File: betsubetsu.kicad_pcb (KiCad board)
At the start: 2 copper layers, 64.5 x 39.4 mm, 24 parts, among them J1 AV IN, J2 VIDEO OUT, J3 AUDIO OUT, T1 TY-250P, U1 THS7374

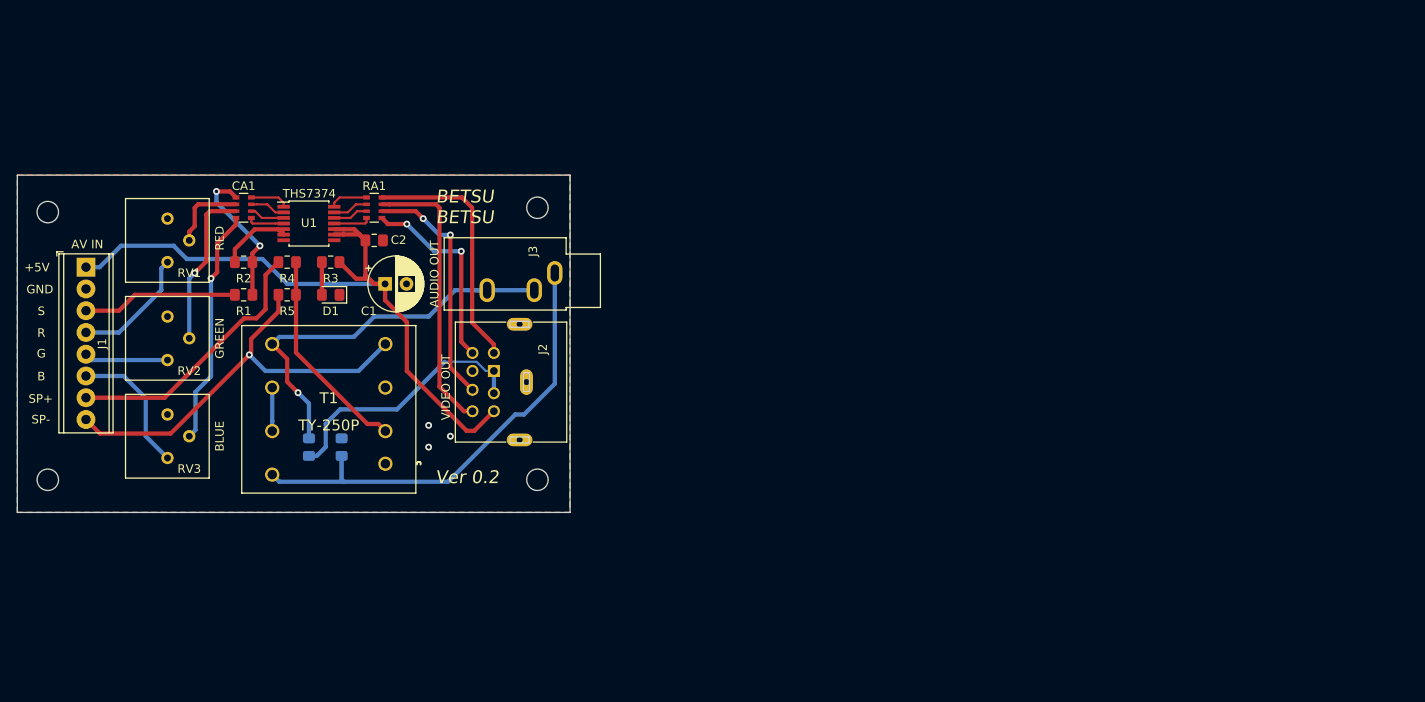
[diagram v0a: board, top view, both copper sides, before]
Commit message: Cleaned up jamma version
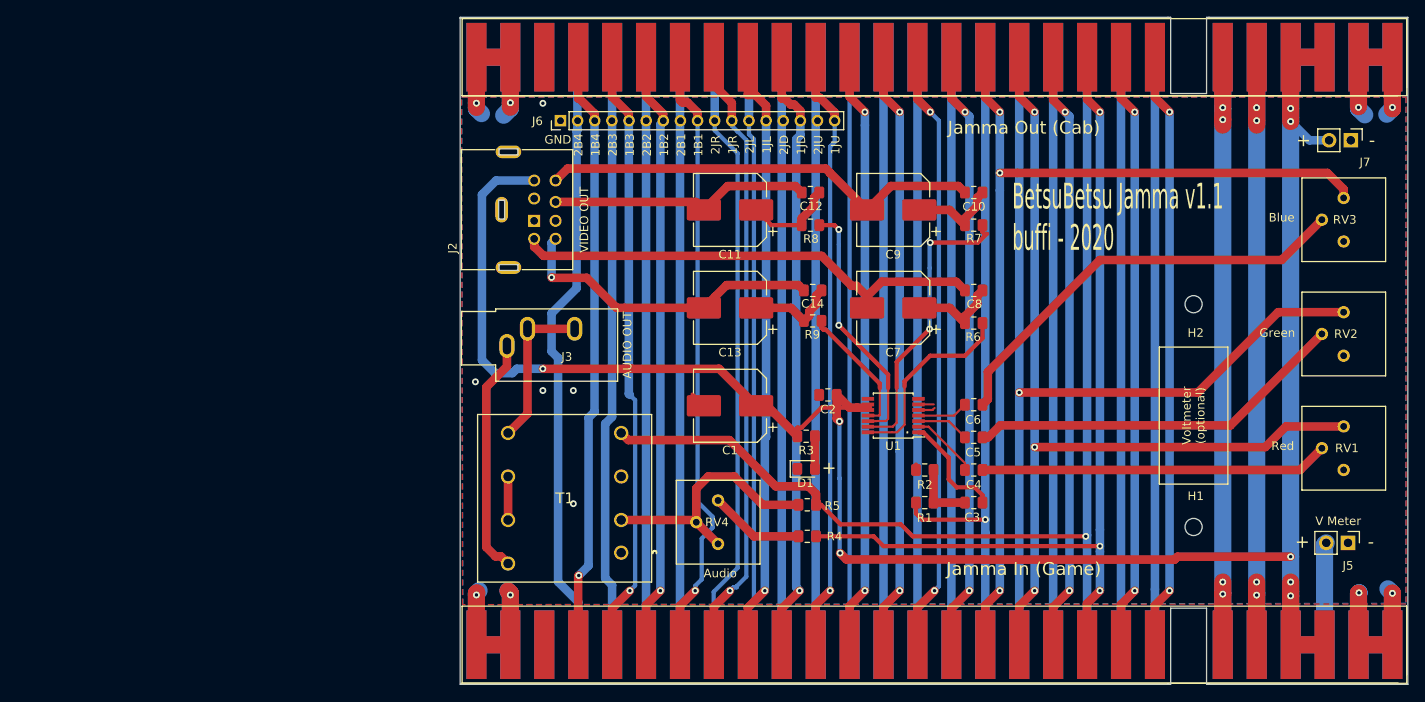
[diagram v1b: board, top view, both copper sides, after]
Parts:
- removed CA1: 0.1uF, Resistor_SMD:R_Array_Convex_4x0603
- removed H3, H4: MountingHole, MountingHole:MountingHole_2.5mm
- removed JMP1: SCART_AUDIO, LED_SMD:LED_0805_2012Metric_Pad1.15x1.40mm_HandSolder
- removed JMP2: AUDIO_GND_TO_GLOBAL_GND, Resistor_SMD:R_0805_2012Metric_Pad1.15x1.40mm_HandSolder
- removed RA1: 75, Resistor_SMD:R_Array_Convex_4x0603
- added C10: 0.1u, Capacitor_SMD:C_0805_2012Metric_Pad1.15x1.40mm_HandSolder, F.Cu at (156.3, 77.0)
- added C11: 470u, Capacitor_SMD:CP_Elec_8x6.7, F.Cu at (127.9, 79.0)
- added C12: 0.1u, Capacitor_SMD:C_0805_2012Metric_Pad1.15x1.40mm_HandSolder, F.Cu at (137.3, 77.0)
- added C13: 470u, Capacitor_SMD:CP_Elec_8x6.7, F.Cu at (127.9, 90.4)
- added C14: 0.1u, Capacitor_SMD:C_0805_2012Metric_Pad1.15x1.40mm_HandSolder, F.Cu at (137.5, 88.4)
- added C3: 0.1u, Capacitor_SMD:C_0805_2012Metric_Pad1.15x1.40mm_HandSolder, F.Cu at (156.3, 113.2)
- added C4: 0.1u, Capacitor_SMD:C_0805_2012Metric_Pad1.15x1.40mm_HandSolder, F.Cu at (156.3, 109.3)
- added C5: 0.1u, Capacitor_SMD:C_0805_2012Metric_Pad1.15x1.40mm_HandSolder, F.Cu at (156.3, 105.5)
- added C6: 0.1u, Capacitor_SMD:C_0805_2012Metric_Pad1.15x1.40mm_HandSolder, F.Cu at (156.3, 101.7)
- added C7: 470u, Capacitor_SMD:CP_Elec_8x6.7, F.Cu at (146.9, 90.4)
- added C8: 0.1u, Capacitor_SMD:C_0805_2012Metric_Pad1.15x1.40mm_HandSolder, F.Cu at (156.3, 88.4)
- added C9: 470u, Capacitor_SMD:CP_Elec_8x6.7, F.Cu at (146.9, 79.0)
- added J4: Jamma In (Game), jamma_connector:JAMMA-56, F.Cu at (150.7, 110.7)
- added J5: V Meter, Connector_PinHeader_2.54mm:PinHeader_1x02_P2.54mm_Vertical, F.Cu at (200.0, 117.9)
- added J6: Conn_01x17, Connector_PinHeader_2.00mm:PinHeader_1x17_P2.00mm_Vertical, F.Cu at (108.1, 68.6)
- added J7: 5V, Connector_PinHeader_2.54mm:PinHeader_1x02_P2.54mm_Vertical, F.Cu at (200.4, 70.9)
- added R6: 75, Resistor_SMD:R_0805_2012Metric_Pad1.15x1.40mm_HandSolder, F.Cu at (156.3, 92.2)
- added R7: 75, Resistor_SMD:R_0805_2012Metric_Pad1.15x1.40mm_HandSolder, F.Cu at (156.3, 80.8)
- added R8: 75, Resistor_SMD:R_0805_2012Metric_Pad1.15x1.40mm_HandSolder, F.Cu at (137.3, 80.8)
- added R9: 75, Resistor_SMD:R_0805_2012Metric_Pad1.15x1.40mm_HandSolder, F.Cu at (137.5, 91.9)
- added RV4: 500, Potentiometer_THT:Potentiometer_Bourns_3386P_Vertical, F.Cu at (126.5, 112.9)
- C1: value 100uF -> 100u; footprint Capacitor_THT:CP_Radial_D6.3mm_P2.50mm -> Capacitor_SMD:CP_Elec_8x6.7
- C2: value 0.1uF -> 0.1u
- H1, H2: value MountingHole -> V METER HOLE (2mm); footprint MountingHole:MountingHole_2.5mm -> MountingHole:MountingHole_2mm
- J1: value AV IN -> Jamma Out (Cab); footprint TerminalBlock_Phoenix:TerminalBlock_Phoenix_MPT-0,5-8-2.54_1x08_P2.54mm_Horizontal -> jamma_connector:JAMMA-56
- J2: footprint MD-80SM:CUI_MD-80SM -> MD-80SM-Connector:MD-80SM
- moved RV3 140.6 mm to (199.5, 77.6), turned to 180 degrees
- moved RV1 138.6 mm to (199.5, 104.3), turned to 180 degrees
- moved RV2 137.4 mm to (199.5, 90.9), turned to 180 degrees
- moved H2 134.2 mm to (182.0, 90.0)
- moved H1 133.9 mm to (182.0, 116.0)
- moved J1 107.3 mm to (150.7, 42.2), turned to 180 degrees
- moved R1 83.1 mm to (150.6, 113.2)
- moved R2 83.1 mm to (150.6, 109.3)
- moved U1 71.8 mm to (146.9, 103.0), turned to 180 degrees
- moved R4 68.6 mm to (136.9, 117.1), turned to 180 degrees
- moved R5 65.5 mm to (136.9, 113.4), turned to 180 degrees
- moved D1 59.1 mm to (136.8, 109.2), turned to 0 degrees
- moved R3 59.1 mm to (136.8, 105.4), turned to 180 degrees
- moved C2 55.9 mm to (139.3, 100.6), turned to 0 degrees
- moved C1 42.7 mm to (127.9, 101.9), turned to 180 degrees
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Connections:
- J1 pad 1: +5V -> GND
- J1 pad 3: SYNC_IN -> +5V
- J1 pad 4: RED_IN -> +5V
- J1 pad 5: GREEN_IN -> -5V
- J1 pad 6: BLUE_IN -> +12V
- J1 pad 8: -AUDIO_IN -> METER1
- J2 pad 1: SCART_AUDIO_OUT -> (no net)
- J2 pad 2: SCART_AUDIO_OUT -> (no net)
- R5 pad 2: Net-(R4-Pad2) -> Net-(R5-Pad2)
- T1 pad 2: Net-(R4-Pad2) -> Net-(R5-Pad2)
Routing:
- net +5V: track 83.0 -> 269.9 mm, vias 0 -> 8
- net GND: track 9.07 -> 142.4 mm, vias 3 -> 13
- net GREEN_IN: track 9.80 -> 110.3 mm, vias 0 -> 1
- net BLUE_IN: track 16.1 -> 111.9 mm, vias 0 -> 3
- net RED_IN: track 14.4 -> 107.1 mm, vias 0 -> 3
- net +12V: track 0.00 -> 80.6 mm, vias 0 -> 4
- net -5V: track 0.00 -> 80.6 mm, vias 0 -> 4
- net -AUDIO_IN: track 49.9 -> 128.8 mm
- net P1_D: track 0.00 -> 74.4 mm, vias 0 -> 1
- net P1_B: track 0.00 -> 73.8 mm, vias 0 -> 1
- net +AUDIO_IN: track 31.4 -> 103.5 mm, vias 0 -> 3
- net P1_A: track 0.00 -> 72.1 mm, vias 0 -> 1
- net P1_RIGHT: track 0.00 -> 72.0 mm, vias 0 -> 1
- net P2_D: track 0.00 -> 71.2 mm
- net P1_DOWN: track 0.00 -> 71.1 mm, vias 0 -> 1
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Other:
- board size 64.5 x 39.4 mm -> 110.6 x 77.9 mm
- board text added: "+"
- board text added: "-"
- board text added: "."
- board text added: "1B1"
- board text added: "1B2"
- board text added: "1B3"
- board text added: "1B4"
- board text added: "1JD"
- board text added: "1JL"
- board text added: "1JR"
- board text added: "1JU"
- board text added: "2B1"
- board text added: "2B2"
- board text added: "2B3"
- board text added: "2B4"
- board text added: "2JD"
- board text added: "2JL"
- board text added: "2JR"
- board text added: "2JU"
- board text added: "Audio"
- board text added: "BetsuBetsu Jamma v1.1 buffi - 2020"
- board text added: "Blue"
- board text added: "Green"
- board text added: "Jamma In (Game)"
- board text added: "Jamma Out (Cab)"
- board text added: "Red"
- board text added: "Voltmeter (optional)"
- board text removed: "+5V"
- board text removed: "B"
- board text removed: "BETSU BETSU"
- board text removed: "BLUE"
- board text removed: "G"
- board text removed: "GREEN"
- board text removed: "R"
- board text removed: "RED"
- board text removed: "S"
- board text removed: "SP+"
- board text removed: "SP-"
- board text removed: "Ver 0.2"
